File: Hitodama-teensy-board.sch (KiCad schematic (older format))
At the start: 16 parts, among them J1 Jack-DC, J2 Conn_01x20_Female, J3 Conn_01x20_Female, J4 Conn_01x20_Female, U4 Teensy3.6

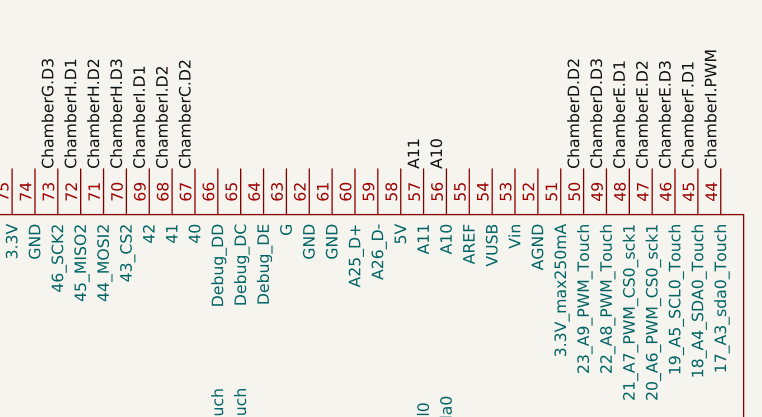
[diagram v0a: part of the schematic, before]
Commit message: trying different routing options teensy board
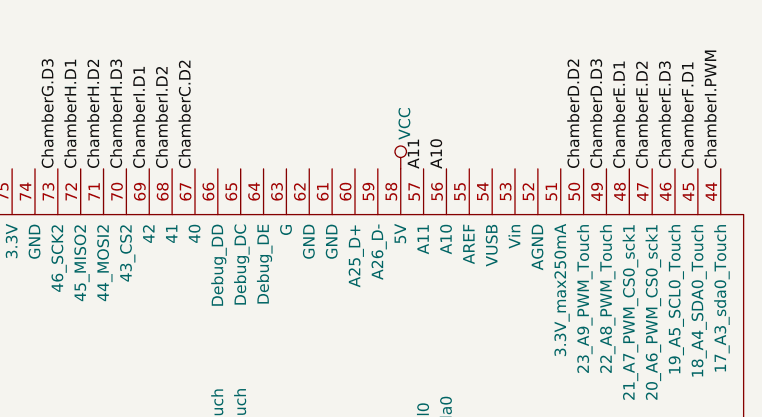
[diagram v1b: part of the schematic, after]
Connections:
- net VCC: now also U4.58 (5V)
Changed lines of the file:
@@
 	0    -1   -1   0
 $EndComp
+$Comp
+L power:VCC #PWR?
+U 1 1 5CE3B325
+P 8200 1600
+F 0 "#PWR?" H 8200 1450 50  0001 C CNN
+F 1 "VCC" V 8218 1727 50  0000 L CNN
+F 2 "" H 8200 1600 50  0001 C CNN
+F 3 "" H 8200 1600 50  0001 C CNN
+	1    8200 1600
+	1    0    0    -1
+$EndComp
 $EndSCHEMATC
